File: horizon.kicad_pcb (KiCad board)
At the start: 4 copper layers, 50 x 100 mm, 261 parts, among them IC1 A3909, J1 Micro_SD_Card_Det1, J10 Conn_01x02_Pin, J11 USB_C_Receptacle_USB2.0_16P, J12 Conn_01x04, J13 1x3 servo, J14 1x3 servo, J15 arming terminal, J16 arming terminal, J17 arming terminal, J18 arming terminal, J19 Screw_Terminal_01x02, J2 Conn_02x03_Counter_Clockwise, J20 Screw_Terminal_01x02, J21 Screw_Terminal_01x02, J22 Screw_Terminal_01x02, J23 USB_C_Receptacle_USB2.0_16P, J24 USB_C_Receptacle_USB2.0_16P, J25 Conn_Coaxial, J3 Conn_Coaxial, J4 H9161TR-ND, J5 Screw_Term, J6 1x3 servo, J7 Conn_02x03_Counter_Clockwise, J8 Conn_02x03_Counter_Clockwise, J9 1x3 servo, Q1 IRLML6402, Q10 IRLML6402, Q11 IRLML6402, Q2 DMG2301L, Q3 IRLML6402, Q4 IRLML6402, Q5 IRLML6402, Q6 IRLML6402, Q7 BSS138, Q8 IRLML6402, Q9 IRLML6402, U1 MMCU, U10 LSM6DS3, U11 BGM220SC12WGA2R, U12 PE4259, U13 LTC4412xS6, U14 TPS61092, U15 AP2112K-3.3, U2 IMU, U3 NMCU, U4 TMCU, U5 LPS22HB, U6 GPS, U7 SX1276, U8 NAND, U9 TPS82130, Y1 Crystal, Y2 32.768kHz, Y4 32MHz

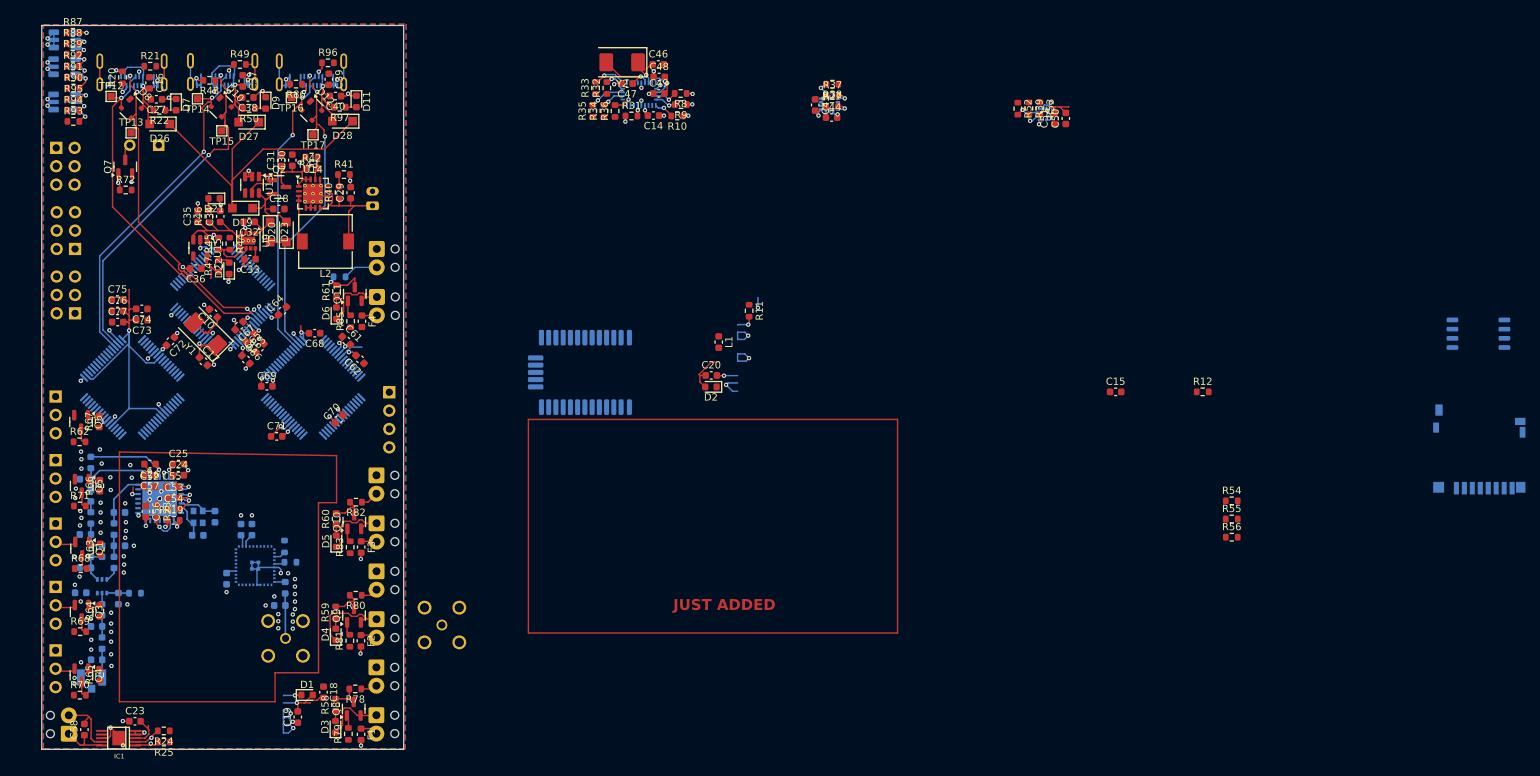
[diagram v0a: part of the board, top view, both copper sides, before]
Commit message: pcb layout done
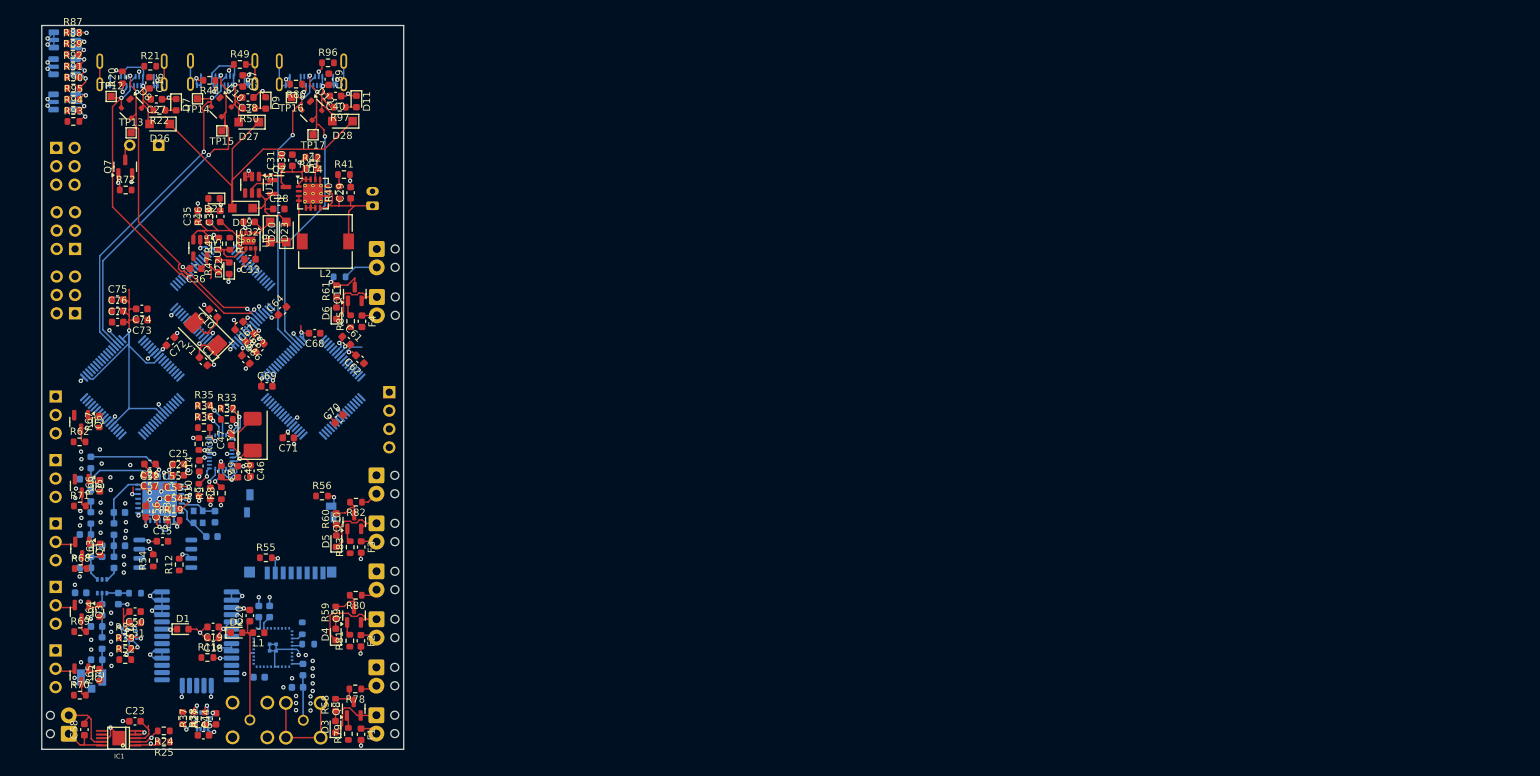
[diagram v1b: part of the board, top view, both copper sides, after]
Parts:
- moved U8 183.9 mm to (92.8, 89.1)
- moved J1 164.7 mm to (110.1, 86.4)
- moved R54 149.2 mm to (91.2, 90.0), turned to 90 degrees
- moved R53 146.0 mm to (87.3, 100.6), turned to 0 degrees
- moved C50 145.5 mm to (88.7, 97.0), turned to 180 degrees
- moved R39 145.5 mm to (87.3, 102.1), turned to 0 degrees
- moved U5 145.0 mm to (88.1, 100.3), turned to -90 degrees
- moved R52 144.9 mm to (87.3, 103.7), turned to 0 degrees
- moved C51 144.9 mm to (88.7, 98.6), turned to 180 degrees
- moved R12 143.4 mm to (94.8, 90.5), turned to 90 degrees
- moved R55 133.5 mm to (106.7, 89.6)
- moved C15 133.3 mm to (92.4, 87.3)
- moved R56 125.8 mm to (114.5, 81.1)
- moved R38 125.4 mm to (95.2, 111.8), turned to -90 degrees
- moved R37 123.2 mm to (96.8, 111.8), turned to 90 degrees
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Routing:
- net GND: track 190.8 -> 216.7 mm, vias 156 -> 158
- net Net-(D2-A): track 10.9 -> 15.4 mm, vias 1 -> 0
- net CS_SD MMCU: track 0.00 -> 3.03 mm, vias 0 -> 1
- net Net-(U11-DECOUPLE): track 1.41 -> 3.97 mm
- net Net-(U8-~{HOLD}/~{RESET}/IO_{3}): track 0.00 -> 2.44 mm, vias 0 -> 1
- net SD_DETECT: track 0.00 -> 2.30 mm, vias 0 -> 1
- net Net-(U8-~{WP}/IO_{2}): track 0.00 -> 2.20 mm, vias 0 -> 1
- net +3.3V: track 121.2 -> 119.2 mm, vias 19 -> 20
- net SX_XTB: track 4.97 -> 5.78 mm
- removed copper zone on B.Cu, net GND
- removed copper zone on F.Cu, net GND
- removed copper zone on In1.Cu, net GND
- removed copper zone on In2.Cu, net GND
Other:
- board text removed: "JUST ADDED"
